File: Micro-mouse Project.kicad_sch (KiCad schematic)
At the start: 10 parts, among them U1 DRV8833PWPR

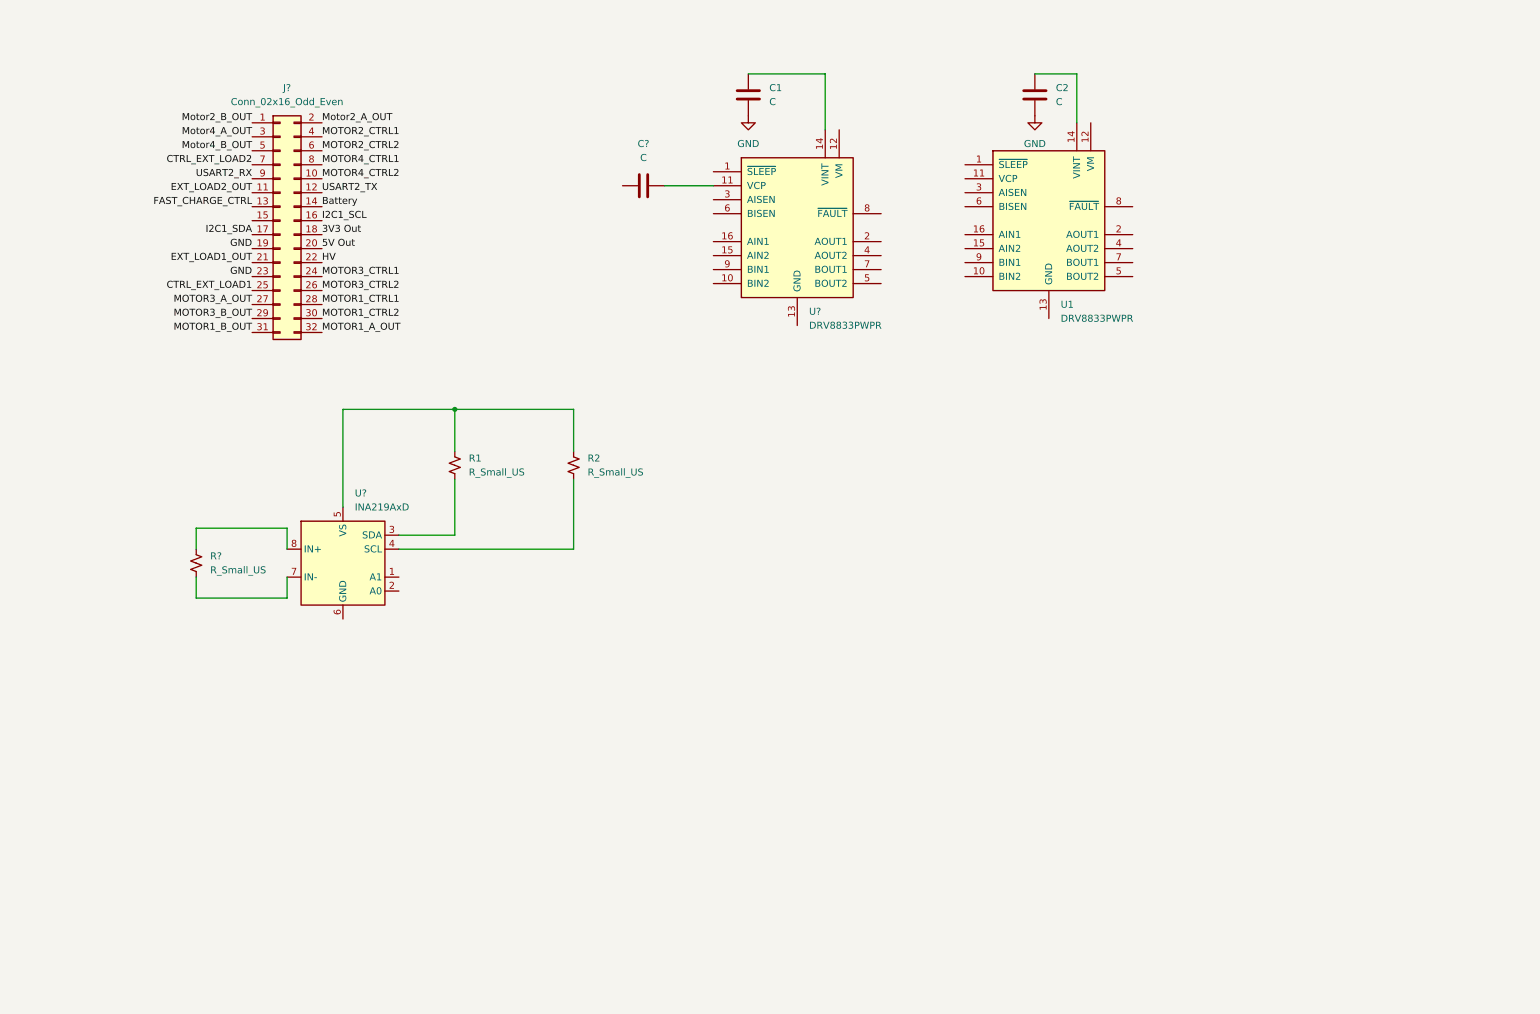
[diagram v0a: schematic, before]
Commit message: Full Schematic
Final draft
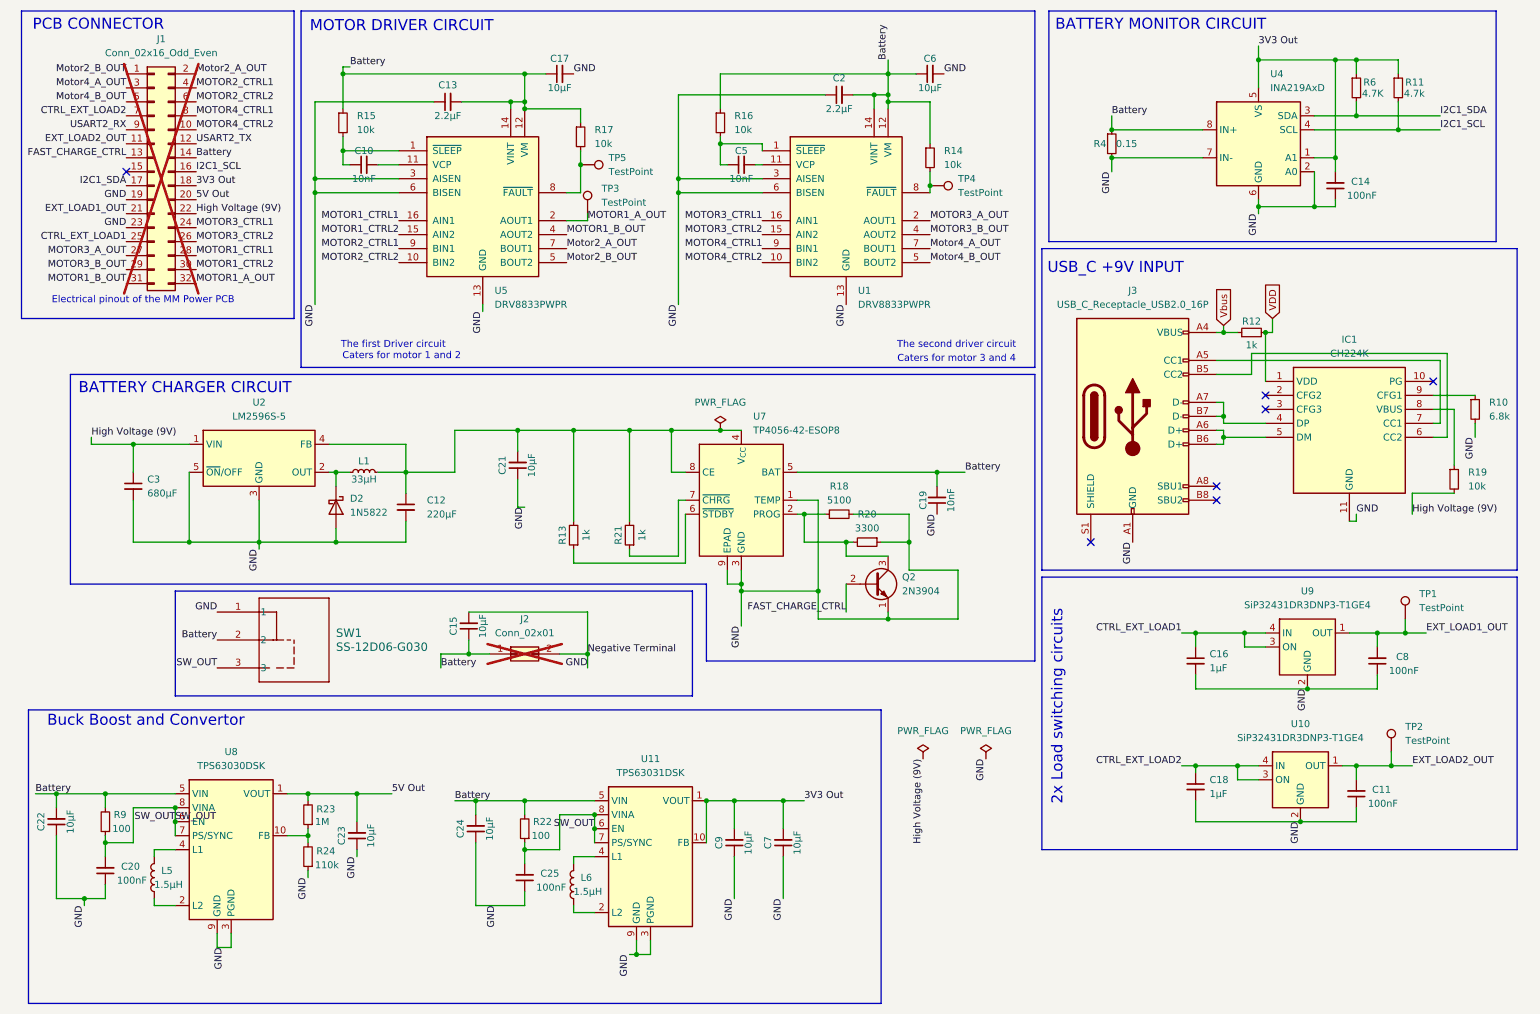
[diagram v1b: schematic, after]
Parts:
- removed C1, C2, C?: C, symbol Device:C
- removed R1, R2, R?: R_Small_US, symbol Device:R_Small_US
- added C10, C19, C5: 10nF, Capacitor_SMD:C_0805_2012Metric_Pad1.18x1.45mm_HandSolder, symbol Device:C_Small
- added C11, C14, C20, C25, C8: 100nF, Capacitor_SMD:C_0402_1005Metric_Pad0.74x0.62mm_HandSolder, symbol Device:C_Small
- added C12: 220μF, Capacitor_SMD:C_1206_3216Metric_Pad1.33x1.80mm_HandSolder, symbol Device:C_Small
- added C13, C2: 2.2μF, Capacitor_SMD:C_0402_1005Metric_Pad0.74x0.62mm_HandSolder, symbol Device:C_Small
- added C15, C17, C21, C22, C23, C24, C6, C7, C9: 10μF, Capacitor_SMD:C_1206_3216Metric_Pad1.33x1.80mm_HandSolder, symbol Device:C_Small
- added C16, C18: 1μF, Capacitor_SMD:C_1206_3216Metric_Pad1.33x1.80mm_HandSolder, symbol Device:C_Small
- added C3: 680μF, Capacitor_THT:C_Radial_D10.0mm_H20.0mm_P5.00mm, symbol Device:C_Small
- added D2: 1N5822, Library:DIO_SS34, symbol Diode:1N5822
- added IC1: CH224K, Library:SOP100P600X180-11N, symbol CH224K:CH224K
- added J2: Conn_02x01, symbol Connector_Generic:Conn_02x01
- added J3: USB_C_Receptacle_USB2.0_16P, Connector_USB:USB_C_Receptacle_GCT_USB4105-xx-A_16P_TopMnt_Horizontal, symbol Connector:USB_C_Receptacle_USB2.0_16P
- added L1: 33μH, Inductor_SMD:L_12x12mm_H4.5mm, symbol Device:L_Small
- added L5, L6: 1.5µH, Inductor_SMD:L_1206_3216Metric_Pad1.22x1.90mm_HandSolder, symbol Device:L
- added Q2: 2N3904, Package_TO_SOT_SMD:SOT-23, symbol Transistor_BJT:2N3904
- added R10: 6.8k, Resistor_SMD:R_0603_1608Metric_Pad0.98x0.95mm_HandSolder, symbol Device:R_Small
- added R11: 4.7k, Resistor_SMD:R_0603_1608Metric_Pad0.98x0.95mm_HandSolder, symbol Device:R_Small
- added R12, R13, R21: 1k, Resistor_SMD:R_1206_3216Metric_Pad1.30x1.75mm_HandSolder, symbol Device:R_Small
- added R14, R15, R16, R17, R19: 10k, Resistor_SMD:R_0805_2012Metric_Pad1.20x1.40mm_HandSolder, symbol Device:R_Small
- added R18: 5100, Resistor_SMD:R_0603_1608Metric, symbol Device:R_Small
- added R20: 3300, Resistor_SMD:R_0603_1608Metric, symbol Device:R_Small
- added R22, R9: 100, Resistor_SMD:R_0805_2012Metric_Pad1.20x1.40mm_HandSolder, symbol Device:R_Small
- added R23: 1M, Resistor_SMD:R_1206_3216Metric_Pad1.30x1.75mm_HandSolder, symbol Device:R_Small
- added R24: 110k, Resistor_SMD:R_0805_2012Metric_Pad1.20x1.40mm_HandSolder, symbol Device:R_Small
- added R4: 0.15, Resistor_SMD:R_1206_3216Metric_Pad1.30x1.75mm_HandSolder, symbol Device:R_Small
- added R6: 4.7K, Resistor_SMD:R_0603_1608Metric_Pad0.98x0.95mm_HandSolder, symbol Device:R_Small
- added SW1: SS-12D06-G030, Library:SS-12D06_GSW, symbol 2025-03-28_06-57-30:SS-12D06-G030
- added TP1, TP2, TP3, TP4, TP5: TestPoint, TestPoint:TestPoint_Pad_D2.0mm, symbol Connector:TestPoint
- added U10: SiP32431DR3DNP3-T1GE4, Library:SON50P120X160X60-5N, symbol Power_Management:SiP32431DR3
- added U11: TPS63031DSK, Package_SON:WSON-10-1EP_2.5x2.5mm_P0.5mm_EP1.2x2mm, symbol Regulator_Switching:TPS63031DSK
- added U2: LM2596S-5, Package_TO_SOT_SMD:TO-263-5_TabPin3, symbol Regulator_Switching:LM2596S-5
- added U7: TP4056-42-ESOP8, Library:SOIC127P600X175-9N, symbol Battery_Management:TP4056-42-ESOP8
- added U8: TPS63030DSK, Package_SON:WSON-10-1EP_2.5x2.5mm_P0.5mm_EP1.2x2mm, symbol Regulator_Switching:TPS63030DSK
- added U9: SiP32431DR3DNP3-T1GE4, Package_TO_SOT_SMD:SOT-363_SC-70-6, symbol Power_Management:SiP32431DR3
- J1: renamed from J?; now not fitted
- U1: footprint Package_SO:HTSSOP-16-1EP_4.4x5mm_P0.65mm_EP3.4x5mm_Mask2.46x2.31mm_ThermalVias -> Library:IC_DRV8833PWPR
- U4: renamed from U?; footprint Package_SO:SOIC-8_3.9x4.9mm_P1.27mm -> Library:SOT65P280X145-8N; LCSC (none) -> C87469
- U5: renamed from U?; footprint Package_SO:HTSSOP-16-1EP_4.4x5mm_P0.65mm_EP3.4x5mm_Mask2.46x2.31mm_ThermalVias -> Library:IC_DRV8833PWPR
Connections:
- net 3V3 Out: now also U4.1 (A1), U4.5 (VS), C14.2, C7.2, C9.2, R11.1, R6.1, U11.1 (VOUT), U11.10 (FB)
- net 5V Out: now also C23.2, R23.2, U8.1 (VOUT)
- net Battery: now also U1.12 (VM), U1.14 (VINT), U4.8 (IN+), U5.12 (VM), U5.14 (VINT), C13.2, C15.1, C17.1, C19.2, C2.2, C22.2, C24.2, C6.1, J2.1 (Pin_1), R14.1, R15.1, R16.1, R17.1, R22.2, R4.1, R9.2, SW1.2, U11.5 (VIN), U7.5 (BAT), U8.5 (VIN)
- net CTRL_EXT_LOAD1: now also C16.1, U9.3 (ON), U9.4 (IN)
- net CTRL_EXT_LOAD2: now also C18.1, U10.3 (ON), U10.4 (IN)
- net EXT_LOAD1_OUT: now also C8.2, TP1.1, U9.1 (OUT)
- net EXT_LOAD2_OUT: now also C11.2, TP2.1, U10.1 (OUT)
- net FAST_CHARGE_CTRL: now also Q2.2 (B)
- net GND: now also U1.13 (GND), U1.17 (GND), U1.3 (AISEN), U1.6 (BISEN), U4.2 (A0), U4.6 (GND), U4.7 (IN-), U5.13 (GND), U5.17 (GND), U5.3 (AISEN), U5.6 (BISEN), C11.1, C12.2, C13.1, C14.1, C15.2, C16.2, C17.2, C18.2, C19.1, C2.1, C20.1, C21.1, C22.1, C23.1, C24.1, C25.1, C3.2, C6.2, C7.1, C8.1, C9.1, D2.2 (A), IC1.11 (GND), J2.2 (Pin_2), J3.A1 (GND), J3.A12 (GND), J3.B1 (GND), J3.B12 (GND), Q2.1 (E), R10.2, R18.2, R20.1, R24.1, R4.2, SW1.1, U10.2 (GND), U10.5 (GND), U11.11 (PGND), U11.3 (PGND), U11.9 (GND), U2.3 (GND), U2.5 (~{ON}/OFF), U7.1 (TEMP), U7.3 (GND), U7.9 (EPAD), U8.11 (PGND), U8.3 (PGND), U8.9 (GND), U9.2 (GND), U9.5 (GND)
- net I2C1_SCL: now also U4.4 (SCL), R11.2
- net I2C1_SDA: now also U4.3 (SDA), R6.2
- net MOTOR1_A_OUT: now also U5.2 (AOUT1), TP3.1
- net MOTOR1_B_OUT: now also U5.4 (AOUT2)
- net MOTOR1_CTRL1: now also U5.16 (AIN1)
- net MOTOR1_CTRL2: now also U5.15 (AIN2)
- net MOTOR2_CTRL1: now also U5.9 (BIN1)
- net MOTOR2_CTRL2: now also U5.10 (BIN2)
- net MOTOR3_A_OUT: now also U1.2 (AOUT1)
- net MOTOR3_B_OUT: now also U1.4 (AOUT2)
- net MOTOR3_CTRL1: now also U1.16 (AIN1)
- net MOTOR3_CTRL2: now also U1.15 (AIN2)
- net MOTOR4_CTRL1: now also U1.9 (BIN1)
- net MOTOR4_CTRL2: now also U1.10 (BIN2)
- net Motor2_A_OUT: now also U5.7 (BOUT1)
- net Motor2_B_OUT: now also U5.5 (BOUT2)
- net Motor4_A_OUT: now also U1.7 (BOUT1)
- net Motor4_B_OUT: now also U1.5 (BOUT2)
- net at U1.1 (~{SLEEP}): now also C5.1, R16.2
- net at U1.11 (VCP): now also C5.2
- net at U1.8 (~{FAULT}): now also R14.2, TP4.1
- net at U5.1 (~{SLEEP}): now also C10.1, R15.2
- net at U5.11 (VCP): now also C10.2
- net at U5.8 (~{FAULT}): now also R17.2, TP5.1
- net HV renamed High Voltage (9V)
- net High Voltage (9V): now also C3.1, R19.2, U2.1 (VIN)
- new net: D2.1 (K), L1.1, U2.2 (OUT)
- new net: C12.1, C21.2, L1.2, R13.2, R21.2, U2.4 (FB), U7.4 (V_{CC}), U7.8 (CE)
- new net: R21.1, U7.7 (~{CHRG})
- new net: Q2.3 (C), R18.1, R20.2, U7.2 (PROG)
- new net: R23.1, R24.2, U8.10 (FB)
- new net: L6.1, U11.2 (L2)
- new net: L6.2, U11.4 (L1)
- new net: IC1.9 (CFG1), R10.1
- new net: L5.1, U8.2 (L2)
- new net: L5.2, U8.4 (L1)
- new net: IC1.7 (CC1), J3.A5 (CC1)
- new net: IC1.5 (DM), J3.A6 (D+), J3.B6 (D+)
- new net: IC1.4 (DP), J3.A7 (D-), J3.B7 (D-)
- new net: IC1.6 (CC2), J3.B5 (CC2)
- new net: IC1.8 (VBUS), R19.1
- new net: R13.1, U7.6 (~{STDBY})
- new net SW_OUT: C20.2, C25.2, R22.1, R9.1, SW1.3, U11.6 (EN), U11.7 (PS/SYNC), U11.8 (VINA), U8.6 (EN), U8.7 (PS/SYNC), U8.8 (VINA)
- new net VDD: IC1.1 (VDD), R12.2
- new net Vbus: J3.A4 (VBUS), J3.A9 (VBUS), J3.B4 (VBUS), J3.B9 (VBUS), R12.1
- no-connect marks 0 -> 7
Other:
- note added: "2x Load switching circuits"
- note added: "BATTERY CHARGER CIRCUIT"
- note added: "BATTERY MONITOR CIRCUIT"
- note added: "Buck Boost and Convertor"
- note added: "Caters for motor 1 and 2"
- note added: "Caters for motor 3 and 4"
- note added: "Electrical pinout of the MM Power PCB"
- note added: "MOTOR DRIVER CIRCUIT"
- note added: "PCB CONNECTOR"
- note added: "The first Driver circuit"
- note added: "The second driver circuit"
- note added: "USB_C +9V INPUT"
- company: (none) -> Universiy of Cape Town
- title: (none) -> GRP 14 POWER SUB-SYSTEM
- moved on the sheet: U1, U4, U5
